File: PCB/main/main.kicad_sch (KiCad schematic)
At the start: 9 parts, among them J1 Conn_01x33_Female, J2 Conn_01x33_Female, J3 Conn_01x33_Female, J4 Conn_01x33_Female

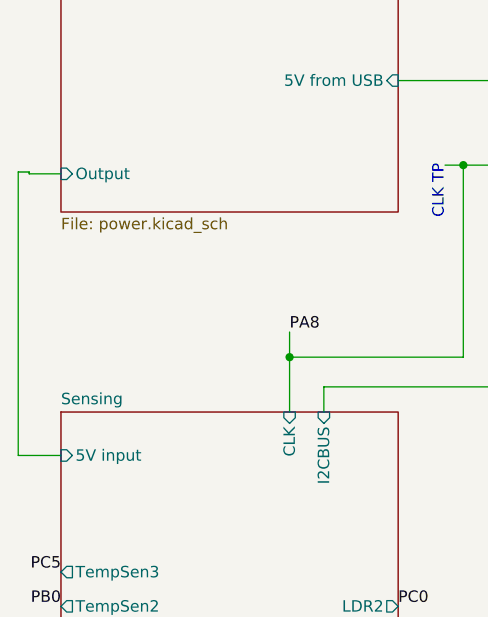
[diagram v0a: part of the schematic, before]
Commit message: updated microcontroller submodule
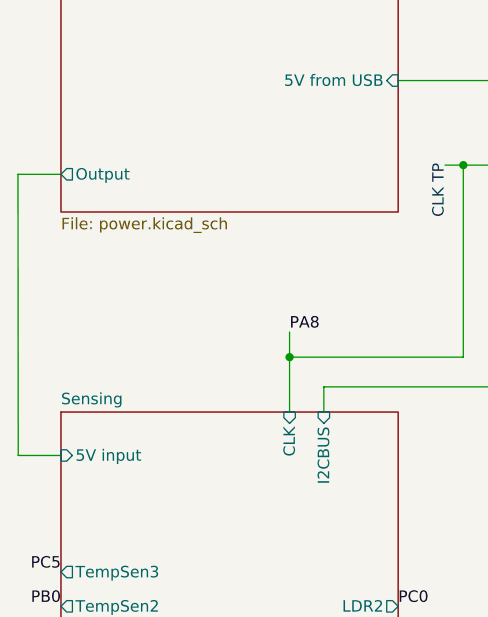
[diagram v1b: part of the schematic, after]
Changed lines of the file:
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@@
-    (stroke (width 0) (type default) (color 0 0 0 0))
-  )
-  (wire (pts (xy 49.8094 68.7832) (xy 49.8094 68.58))
     (stroke (width 0) (type default) (color 0 0 0 0))
   )
@@
     (stroke (width 0) (type default) (color 0 0 0 0))
   )
-  (wire (pts (xy 49.8094 68.58) (xy 48.5902 68.58))
+  (wire (pts (xy 48.5648 68.834) (xy 53.34 68.834))
     (stroke (width 0) (type default) (color 0 0 0 0))
   )
@@
     (stroke (width 0) (type default) (color 0 0 0 0))
   )
-  (wire (pts (xy 48.5902 68.58) (xy 48.5902 100.076))
-    (stroke (width 0) (type default) (color 0 0 0 0))
-  )
-  (wire (pts (xy 53.34 68.7832) (xy 49.8094 68.7832))
+  (wire (pts (xy 48.5648 68.834) (xy 48.5902 100.076))
     (stroke (width 0) (type default) (color 0 0 0 0))
   )
@@
       (effects (font (size 1.27 1.27)) (justify right))
     )
-    (pin "Output" input (at 53.34 68.7832 180)
+    (pin "Output" output (at 53.34 68.834 180)
       (effects (font (size 1.27 1.27)) (justify left))
     )
@@
       (reference "R18") (unit 1) (value "4K7") (footprint "Resistor_SMD:R_0201_0603Metric")
     )
+    (path "/59b42903-2dc7-4011-ab5b-d7b81bd233c3/96763a51-1ff4-43a2-9943-9546ef8a9b30"
+      (reference "R19") (unit 1) (value "0") (footprint "Resistor_SMD:R_0201_0603Metric")
+    )
+    (path "/59b42903-2dc7-4011-ab5b-d7b81bd233c3/7f0b7a33-2a31-4936-ad80-c56d49591622"
+      (reference "R20") (unit 1) (value "0") (footprint "Resistor_SMD:R_0201_0603Metric")
+    )
     (path "/59b42903-2dc7-4011-ab5b-d7b81bd233c3/ead29cac-b026-47a5-966a-8205558ed08d"

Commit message: updated gerbers and finalized PCB
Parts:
- J2, J3: Alt_LCSC C12345 (example) -> (none); LCSC C1234 (example) -> (none)
- TP1, TP2, TP3, TP4, TP5: Populate (none) -> DNP
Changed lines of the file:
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@@
+      (effects (font (size 1.27 1.27)) hide)
+    )
+    (property "Populate" "DNP" (id 4) (at 204.978 148.59 0)
       (effects (font (size 1.27 1.27)) hide)
     )
@@
       (effects (font (size 1.27 1.27)) hide)
     )
+    (property "Populate" "DNP" (id 4) (at 204.47 134.366 0)
+      (effects (font (size 1.27 1.27)) hide)
+    )
     (pin "1")
   )
@@
       (effects (font (size 1.27 1.27)) hide)
     )
+    (property "Populate" "DNP" (id 4) (at 204.47 141.478 0)
+      (effects (font (size 1.27 1.27)) hide)
+    )
     (pin "1")
   )
@@
       (effects (font (size 1.27 1.27)) hide)
     )
-    (property "LCSC" "C1234 (example)" (id 4) (at 224.155 64.77 0)
+    (property "LCSC" "" (id 4) (at 224.155 64.77 0)
       (effects (font (size 1.27 1.27)) hide)
     )
@@
       (effects (font (size 1.27 1.27)) hide)
     )
-    (property "Alt_LCSC" "C12345 (example)" (id 6) (at 224.155 64.77 0)
+    (property "Alt_LCSC" "" (id 6) (at 224.155 64.77 0)
       (effects (font (size 1.27 1.27)) hide)
     )
@@
       (effects (font (size 1.27 1.27)) hide)
     )
+    (property "Populate" "DNP" (id 4) (at 204.216 127.762 0)
+      (effects (font (size 1.27 1.27)) hide)
+    )
     (pin "1")
   )
@@
       (effects (font (size 1.27 1.27)) hide)
     )
-    (property "LCSC" "C1234 (example)" (id 4) (at 243.205 64.77 0)
+    (property "LCSC" "" (id 4) (at 243.205 64.77 0)
       (effects (font (size 1.27 1.27)) hide)
     )
@@
       (effects (font (size 1.27 1.27)) hide)
     )
-    (property "Alt_LCSC" "C12345 (example)" (id 6) (at 243.205 64.77 0)
+    (property "Alt_LCSC" "" (id 6) (at 243.205 64.77 0)
       (effects (font (size 1.27 1.27)) hide)
     )
@@
       (effects (font (size 1.27 1.27)) hide)
     )
+    (property "Populate" "DNP" (id 4) (at 204.216 121.666 0)
+      (effects (font (size 1.27 1.27)) hide)
+    )
     (pin "1")
   )
@@
     )
     (path "/59b42903-2dc7-4011-ab5b-d7b81bd233c3/c322890e-14c1-46f5-b267-f55221ee900f"
-      (reference "C4") (unit 1) (value "CT41G-0402-2X1-16V-0.1μF-K(N)") (footprint "Capacitor_SMD:C_0201_0603Metric")
+      (reference "C4") (unit 1) (value "0.1μF") (footprint "Capacitor_SMD:C_0201_0603Metric")
     )
     (path "/d15c8919-7ccc-44b2-8fc4-b04c1b47b6fa/7312d6c1-286a-4148-a5c3-52b226791586"
@@
     )
     (path "/d15c8919-7ccc-44b2-8fc4-b04c1b47b6fa/2cb653ae-a486-4999-8f63-2cc2ca83bff5"
-      (reference "L1") (unit 1) (value "MLP2012V4R7MT0S1") (footprint "Inductor_SMD:L_0805_2012Metric")
+      (reference "L1") (unit 1) (value "MLP2012V4R7MT0S1") (footprint "3088HAT:INDC2012X87N")
     )
     (path "/cf6c12a4-3d95-473d-bafe-8be3892a84e9/90369ffc-d873-4b5f-ab01-ddf820143b6f"
@@
     )
     (path "/d15c8919-7ccc-44b2-8fc4-b04c1b47b6fa/768374ff-fcd3-47db-8a39-62497a662f1b"
-      (reference "R1") (unit 1) (value "1650") (footprint "Resistor_SMD:R_0201_0603Metric")
+      (reference "R1") (unit 1) (value "1800") (footprint "Resistor_SMD:R_0201_0603Metric")
     )
     (path "/d15c8919-7ccc-44b2-8fc4-b04c1b47b6fa/625263f4-7654-4012-90f5-ccfddd1120cf"
@@
     )
     (path "/d15c8919-7ccc-44b2-8fc4-b04c1b47b6fa/ced83566-388d-4f99-be31-41bdc857545a"
-      (reference "R3") (unit 1) (value "100") (footprint "Resistor_SMD:R_0201_0603Metric")
+      (reference "R3") (unit 1) (value "100ohms") (footprint "Resistor_SMD:R_0201_0603Metric")
     )
     (path "/d15c8919-7ccc-44b2-8fc4-b04c1b47b6fa/a6859af7-c2bb-496d-bf21-a4a555131e66"
@@
     )
     (path "/d15c8919-7ccc-44b2-8fc4-b04c1b47b6fa/842d48ad-8b90-46f9-8160-46c5ec76f179"
-      (reference "R5") (unit 1) (value "1000") (footprint "Resistor_SMD:R_0201_0603Metric")
+      (reference "R5") (unit 1) (value "1200") (footprint "Resistor_SMD:R_0201_0603Metric")
     )
     (path "/d15c8919-7ccc-44b2-8fc4-b04c1b47b6fa/6fe27d7a-8728-4218-b48e-6f66377c607f"
